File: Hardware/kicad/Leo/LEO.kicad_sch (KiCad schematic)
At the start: 75 parts, among them J1 Conn_01x02, J2 Screw_Terminal_01x04, J4 Conn_01x02, J5 Conn_01x05, J6 Screw_Terminal_01x05, J7 USB_B_Micro, Q1 AO3401A, Q2 AO3400A, Q3 AO3401A, Q4 AO3400A, Q5 AO3400A, Q9 AO3400A, U2 BMI088, U3 BMP388, U4 LIS3MDLTR, U5 ADXL375BCCZ-RL7, U6 RT9013-33GB_C19268157, U8 RP2040, U9 W25Q128JVS, X2 SX1M12.000M10F30TNN

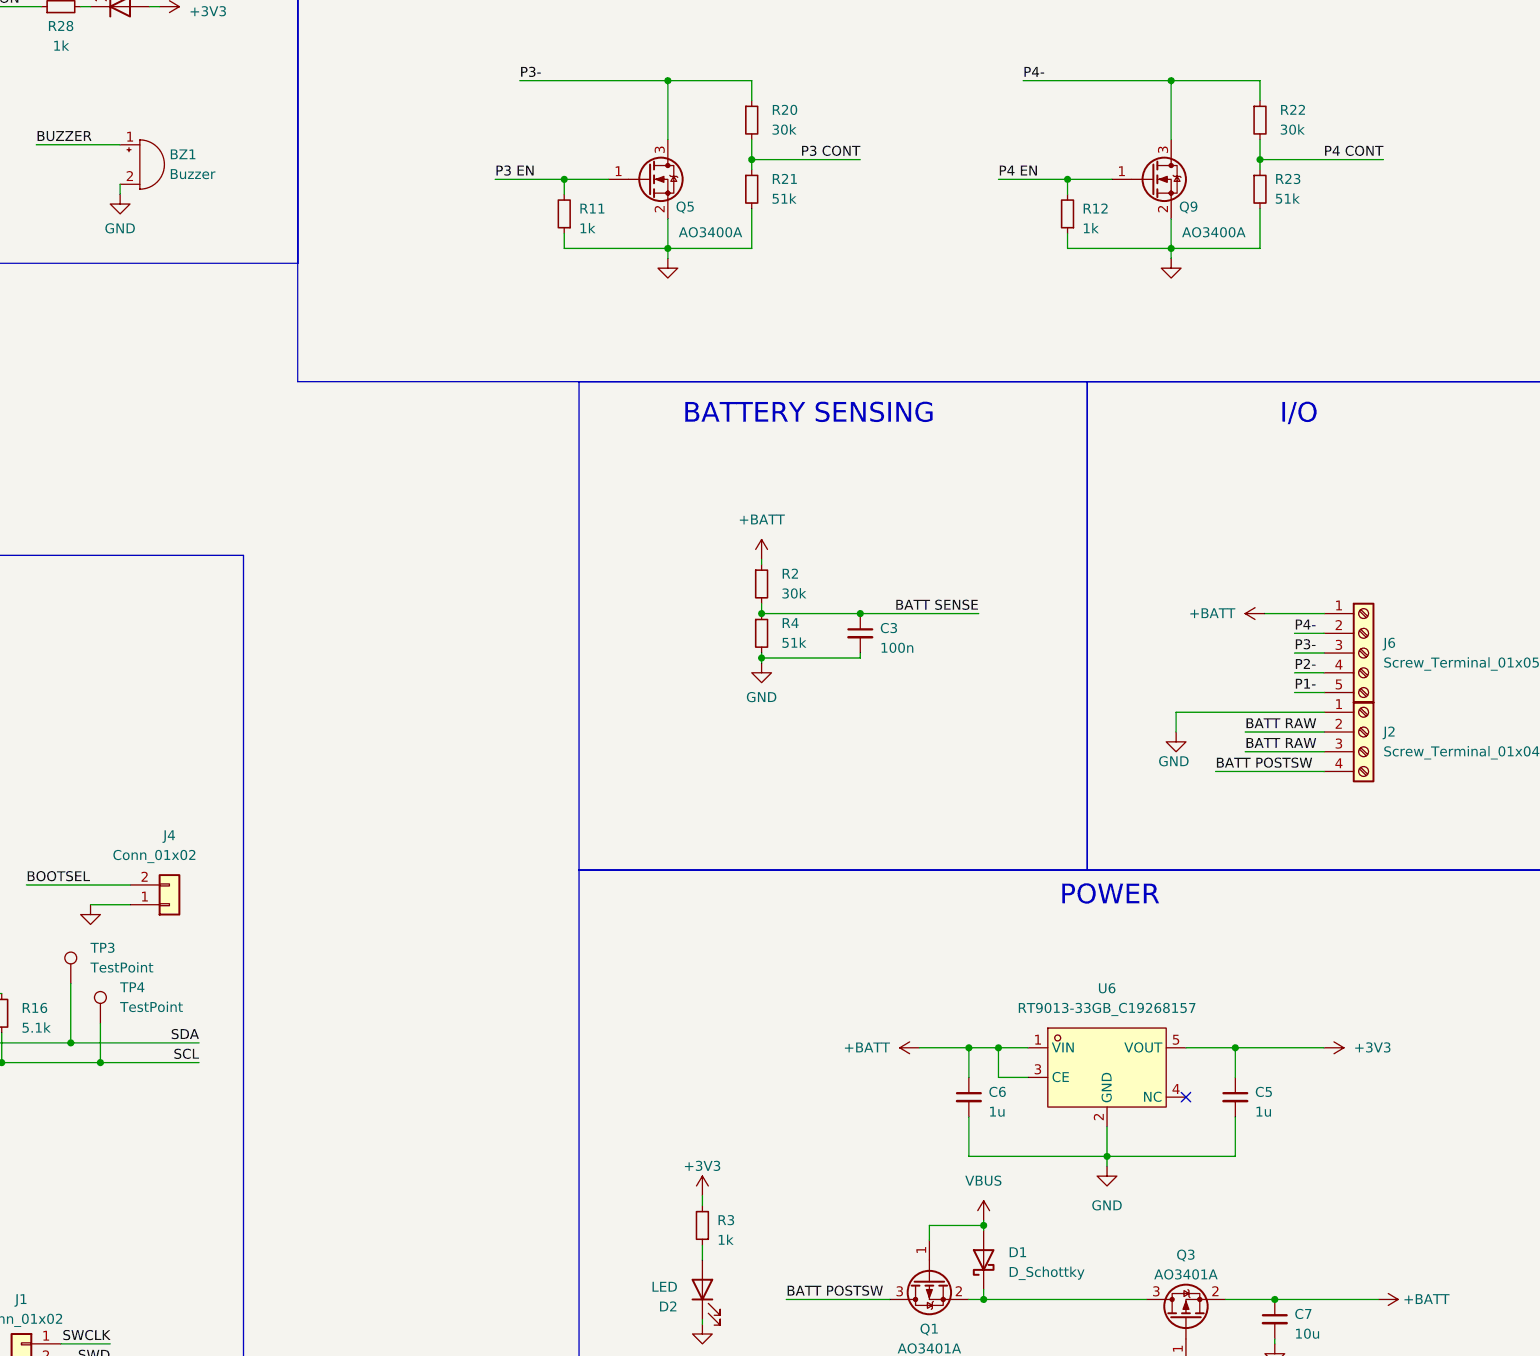
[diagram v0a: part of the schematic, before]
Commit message: things
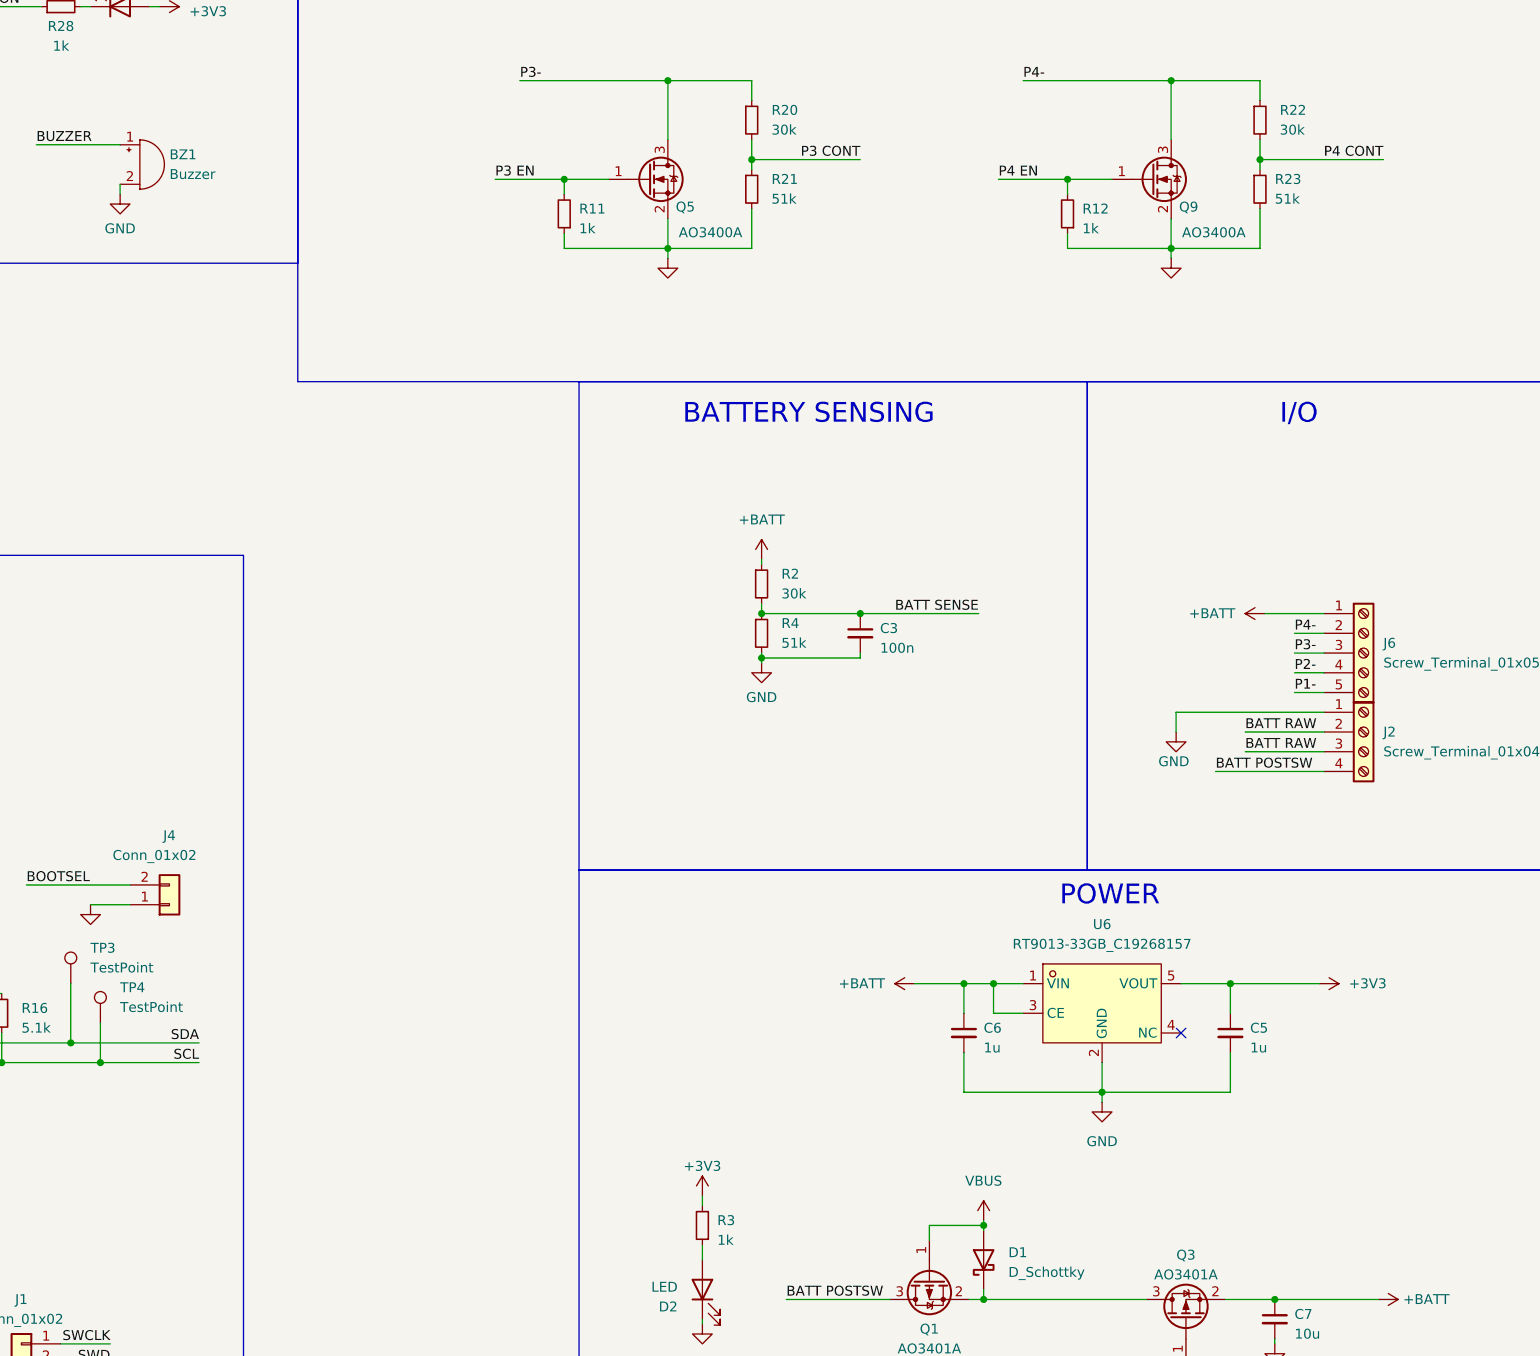
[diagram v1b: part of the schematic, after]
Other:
- moved on the sheet: C5, C6, U6
